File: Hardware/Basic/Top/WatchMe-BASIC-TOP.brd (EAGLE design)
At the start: 38 x 38 mm, 65 parts, among them SW1 SWITCH.MOM, SW2 SWITCH.MOM, U2 NRF52832_MODULE_MDBT42, U4 PCF8523, U5 FT231XS

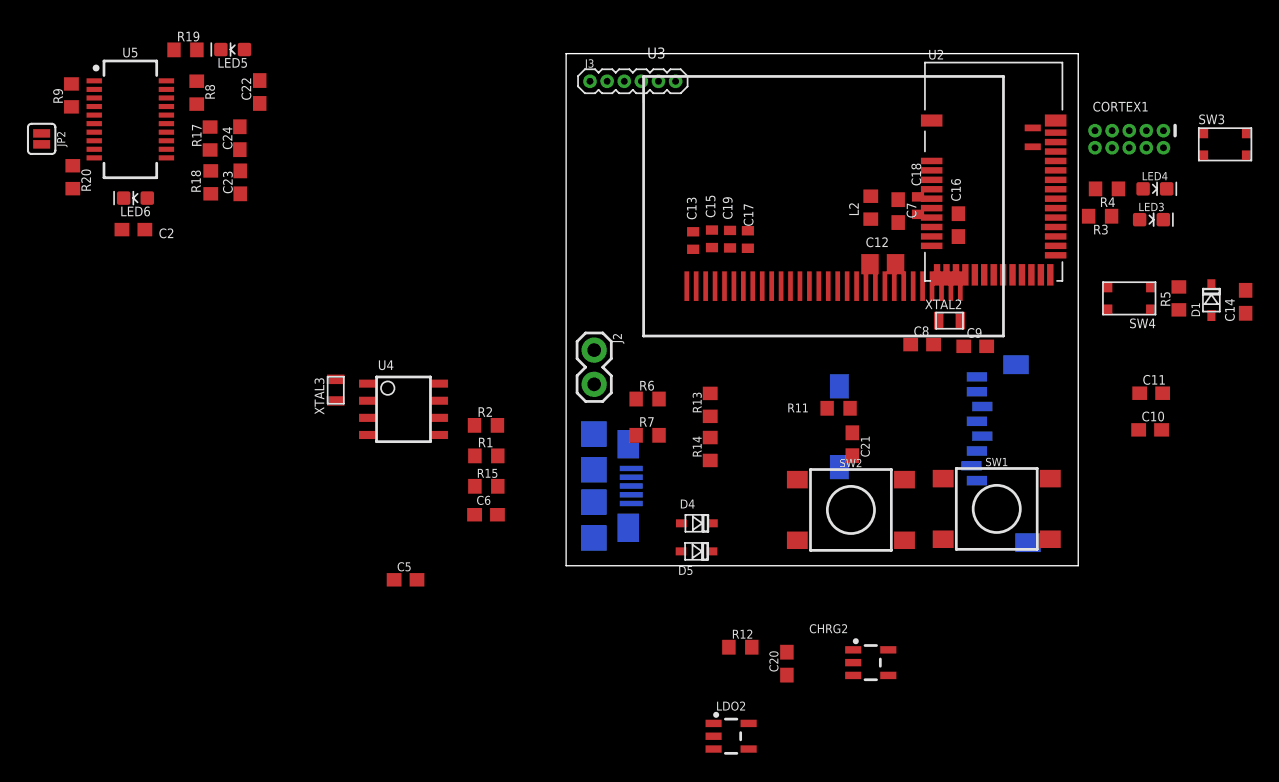
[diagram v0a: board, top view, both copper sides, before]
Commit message: continuin top board work
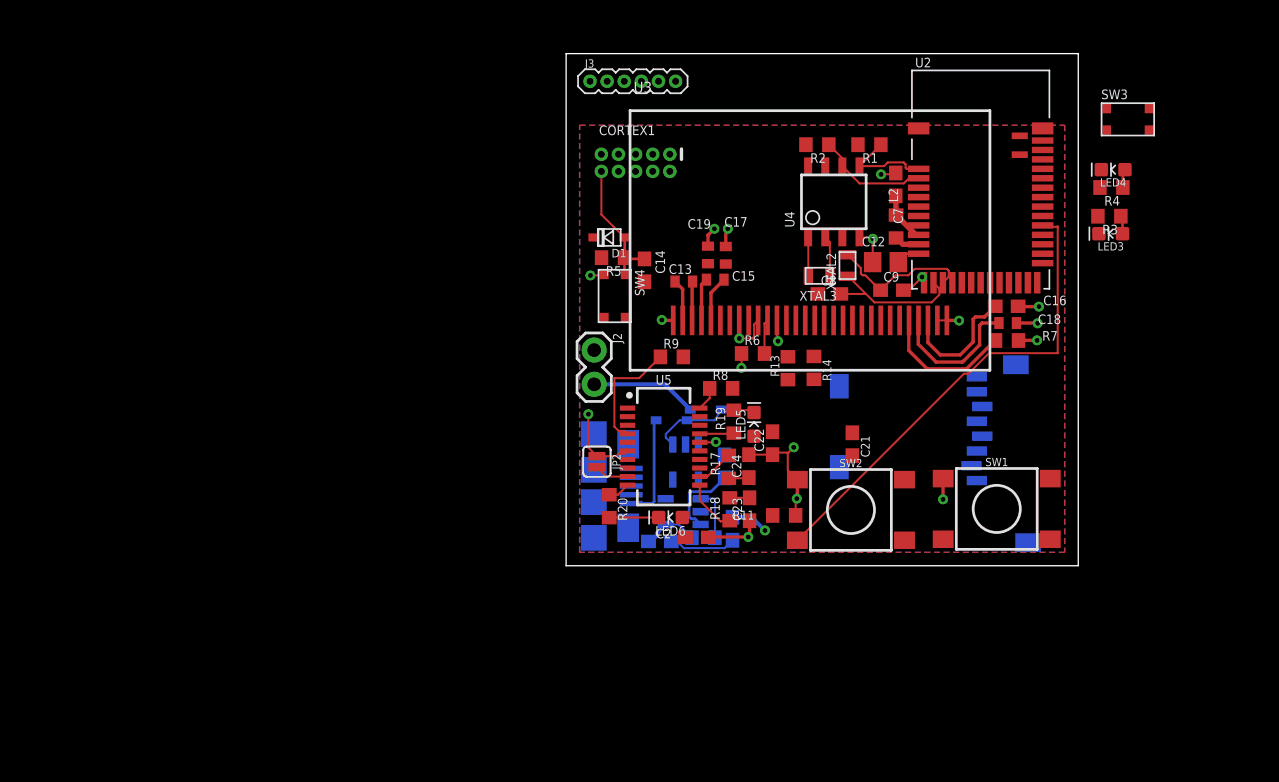
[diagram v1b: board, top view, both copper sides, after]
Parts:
- removed C10, C11: 300p, LinnesLab-Passives:C0603
- removed R15: 100k, LinnesLab-Passives:R0603
- moved R19 49.2 mm to (12.4, 10.7), turned to 90 degrees
- moved R9 48.6 mm to (7.85, 15.5), turned to 0 degrees
- moved JP2 47.7 mm to (2.29, 7.72)
- moved LED5 47.6 mm to (13.9, 10.5), turned to 90 degrees
- moved C2 47.6 mm to (9.70, 2.11), turned to 0 degrees
- moved R20 46.7 mm to (3.20, 4.42)
- moved U5 46.4 mm to (7.24, 8.84)
- moved LED6 46.2 mm to (7.75, 3.58)
- moved C22 46.1 mm to (15.3, 9.09)
- moved R17 45.5 mm to (12.1, 7.34)
- moved R18 45.5 mm to (12.1, 4.19)
- moved C24 44.9 mm to (13.6, 7.39)
- moved D1 44.9 mm to (3.20, 24.4), turned to 180 degrees
- moved C23 44.9 mm to (13.6, 4.19)
- moved R8 44.7 mm to (11.5, 13.2), turned to 0 degrees
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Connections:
- net 3.3V: no longer R15.2
- net GND: no longer C10.2, C11.2, R15.1, SW1.B2, SW2.B2
- net P0.09/NFC1: no longer C11.1
- net P0.10/NFC2: no longer C10.1
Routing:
- net GND: track 0.00 -> 49.8 mm, vias 0 -> 20
- net D15/SW2: track 0.00 -> 35.7 mm
- net VLIPO: track 0.00 -> 13.8 mm
- net N$6: track 0.00 -> 10.9 mm
- net N$4: track 0.00 -> 10.8 mm
- net VIN: track 0.00 -> 10.4 mm
- net N$15: track 0.00 -> 10.4 mm
- net N$2: track 0.00 -> 10.1 mm
- net RESET: track 0.00 -> 9.97 mm
- net N$13: track 0.00 -> 9.50 mm
- net RXD.FT: track 0.00 -> 8.97 mm
- net SCL: track 0.00 -> 8.36 mm
- net V_USB: track 0.00 -> 7.84 mm
- net SDA: track 0.00 -> 7.11 mm
- net 3.3V: track 0.00 -> 4.59 mm, vias 0 -> 1
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- added copper zone on layer 1, net 9V
- added copper zone on layer 16, net GND

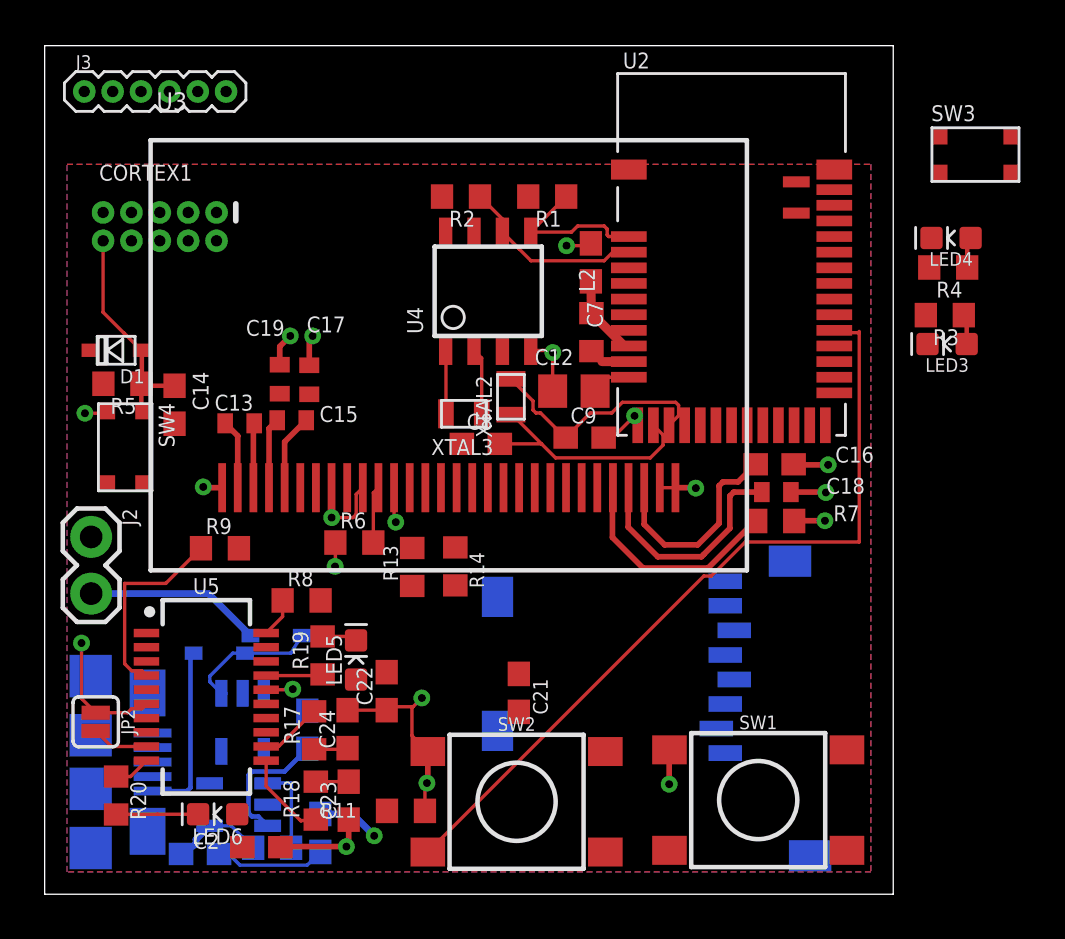
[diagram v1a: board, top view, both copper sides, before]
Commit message: updated top board, still pretty chaotic
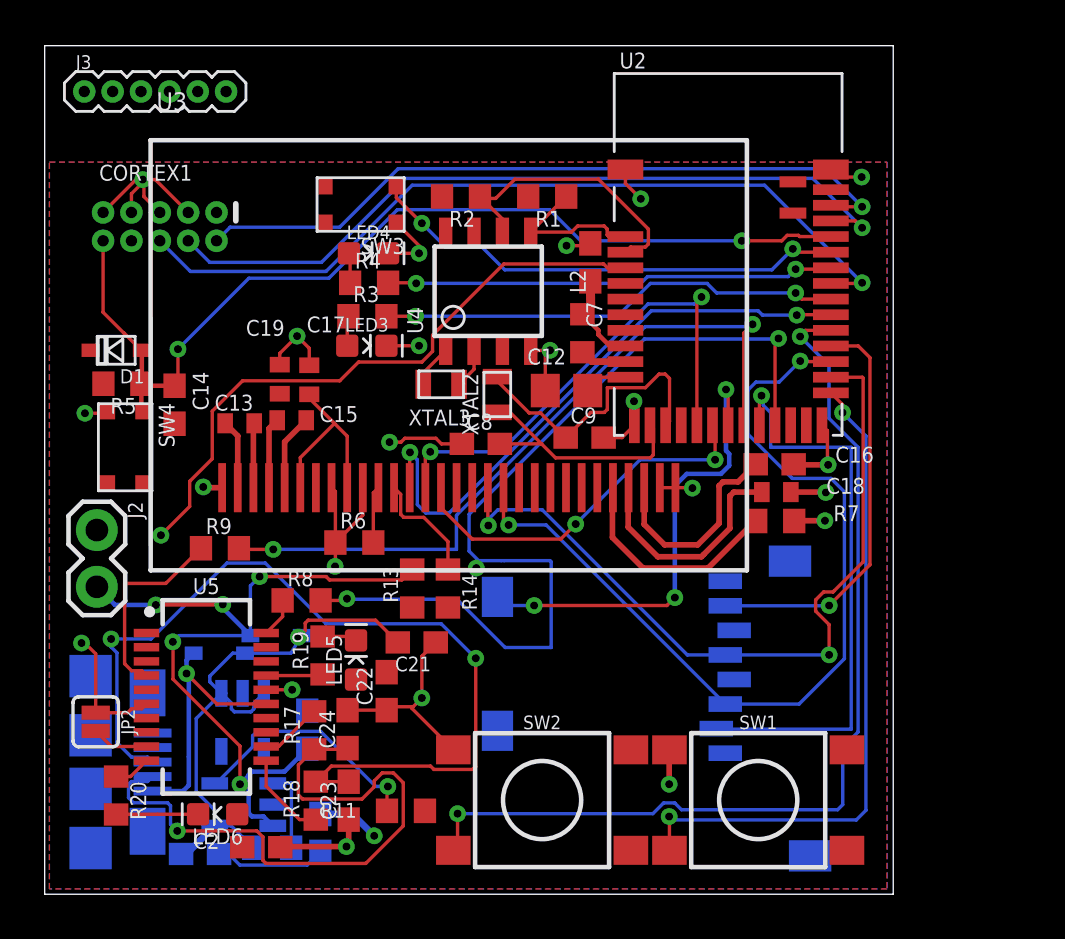
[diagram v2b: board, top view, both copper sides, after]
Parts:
- moved SW3 27.6 mm to (14.1, 30.9), turned to 180 degrees
- moved LED4 26.1 mm to (14.5, 28.7), turned to 0 degrees
- moved LED3 26.0 mm to (14.4, 24.6), turned to 0 degrees
- moved R4 25.9 mm to (14.5, 27.4), turned to 0 degrees
- moved R3 25.9 mm to (14.5, 25.9), turned to 0 degrees
- moved C21 5.10 mm to (16.7, 11.3), turned to 180 degrees
- moved XTAL3 1.67 mm to (17.8, 22.8)
- moved SW2 1.15 mm to (22.3, 4.22)
- moved R14 1.04 mm to (18.1, 13.7)
- moved R13 0.97 mm to (16.5, 13.7)
- moved XTAL2 0.62 mm to (20.3, 22.4)
- moved L2 0.41 mm to (24.1, 25.1)
- moved J2 0.40 mm to (2.34, 16.3)
- moved C12 0.33 mm to (23.4, 22.6)
- moved CHRG2 0.23 mm to (8.92, 4.01)
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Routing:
- net RXD.NRF: track 0.00 -> 41.7 mm, vias 0 -> 2
- net MOSI: track 0.00 -> 40.1 mm, vias 0 -> 2
- net USB+: track 1.47 -> 40.1 mm, vias 0 -> 2
- net SWO: track 0.00 -> 36.8 mm, vias 0 -> 1
- net SCK: track 0.00 -> 35.4 mm, vias 0 -> 2
- net SWCLK: track 0.00 -> 34.6 mm, vias 0 -> 1
- net RESET: track 9.97 -> 44.2 mm, vias 0 -> 2
- net TXD.NRF: track 0.00 -> 32.8 mm, vias 0 -> 2
- net SWDIO: track 0.00 -> 32.4 mm, vias 0 -> 1
- net GND: track 49.8 -> 80.1 mm, vias 20 -> 23
- net D11/SW1: track 0.00 -> 29.9 mm, vias 0 -> 2
- net D27/CHRG.STATUS: track 3.97 -> 32.0 mm, vias 0 -> 1
- net USB-: track 1.52 -> 28.5 mm, vias 0 -> 1
- net D16/CS.OLED: track 0.00 -> 26.6 mm, vias 0 -> 2
- net D7/SD.CS: track 0.00 -> 26.1 mm, vias 0 -> 1
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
